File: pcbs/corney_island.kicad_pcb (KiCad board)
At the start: 2 copper layers, 130.3 x 85.7 mm, 122 parts

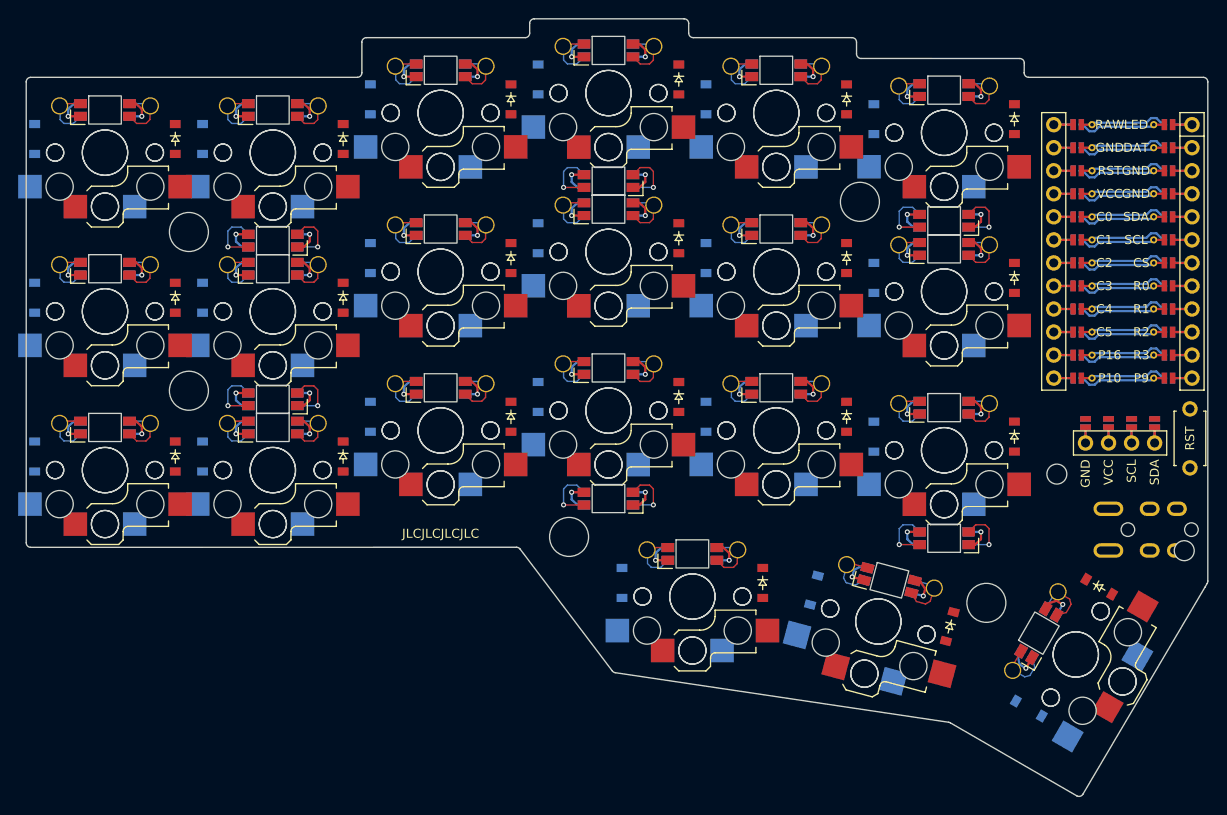
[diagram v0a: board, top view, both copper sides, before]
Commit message: Tralalala
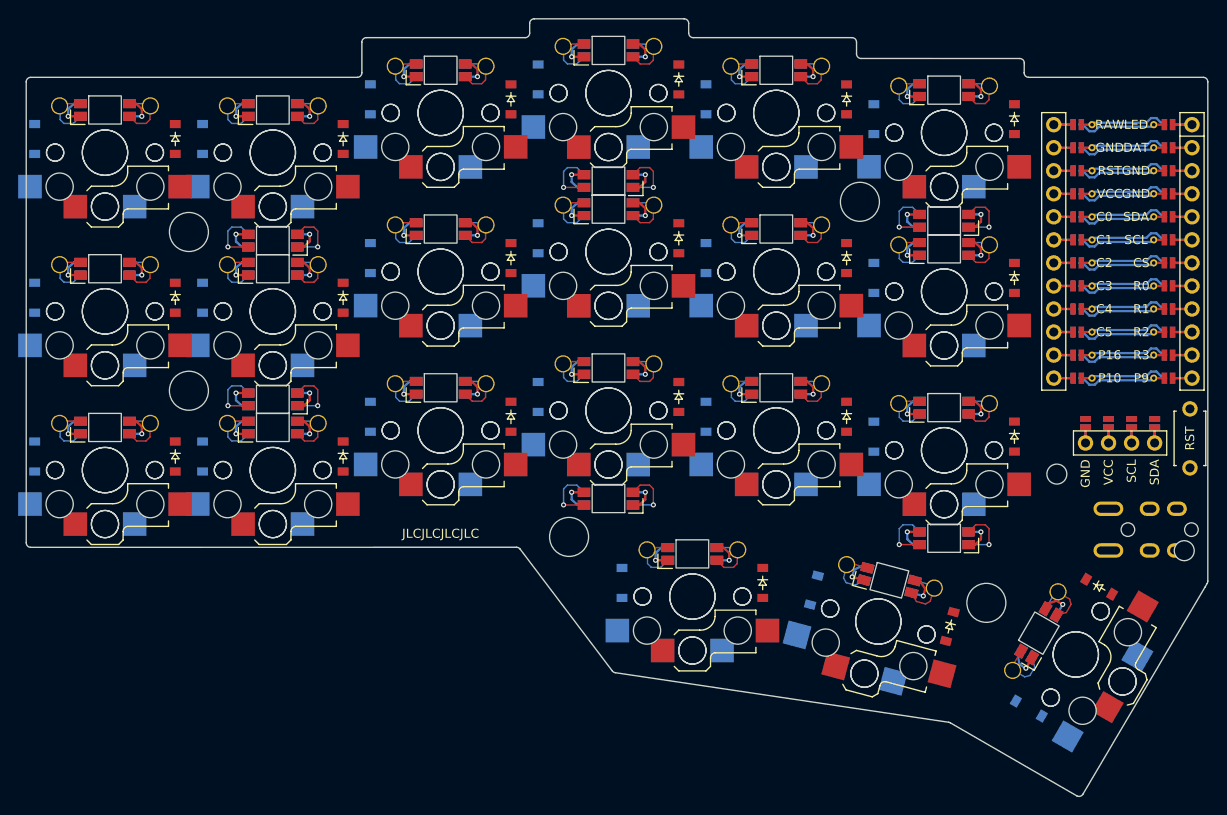
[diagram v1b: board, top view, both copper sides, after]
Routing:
- net (no net): track 0.00 -> 333.1 mm
- net GND: track 130.3 -> 101.4 mm
- net C3: track 9.64 -> 0.00 mm
- net C1: track 9.64 -> 0.00 mm
- net RAW: track 9.64 -> 0.00 mm
- net RST: track 9.64 -> 0.00 mm
- net C5: track 9.64 -> 0.00 mm
- net C4: track 9.64 -> 0.00 mm
- net P16: track 9.64 -> 0.00 mm
- net P10: track 9.64 -> 0.00 mm
- net C2: track 9.64 -> 0.00 mm
- net C0: track 9.64 -> 0.00 mm
- net VCC: track 111.0 -> 101.4 mm
- net SDA: track 9.63 -> 0.00 mm
- net R3: track 9.63 -> 0.00 mm
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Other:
- outline, holes or cut-outs redrawn
